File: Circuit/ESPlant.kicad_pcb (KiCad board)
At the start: 2 copper layers, 97 x 77.5 mm, 68 parts, among them P1 SOIL, P101 CONN_DIGITAL, P102 CONN_ANALOG, P103 CONN_SERIAL, P104 CONN_I2C, P105 SOLAR, P106 USB_5PIN_SHELL, P109 CONN_PWR, P110 CONN_01X05, P111 UV, P112 TEMP, P113 NEOPIXEL, P114 PIR, Q101 FDN340P, Q201 FDN340P, Q202 FDN340P, Q203 FDN340P, SW101 RESET, SW102 PRGM, SW103 RESET, U101 STM32F042F, U103 ESP-12E, U201 CN3063, U202 MCP6002, U301 BME280, U302 ADXL345

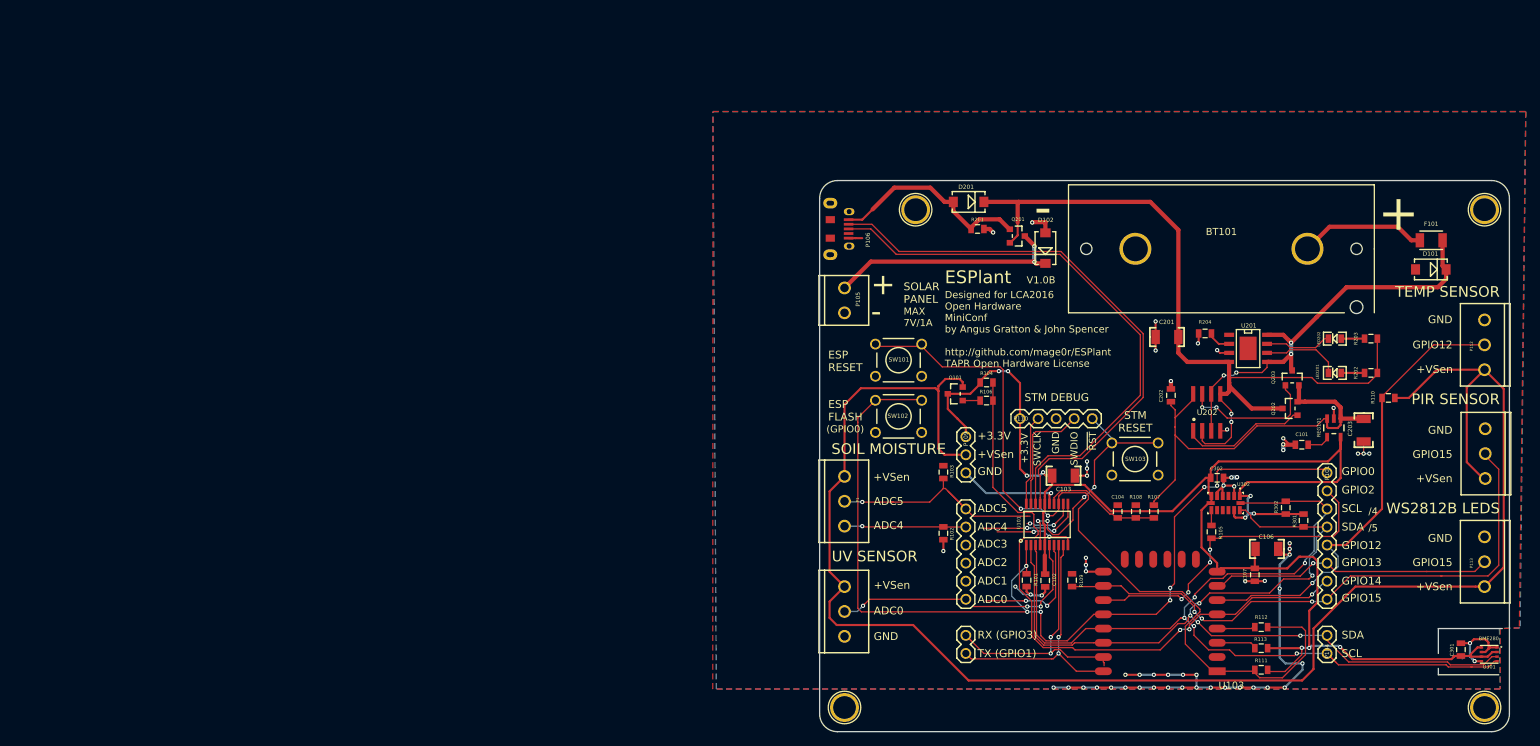
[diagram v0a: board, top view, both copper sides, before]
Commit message: Second go at a layout.
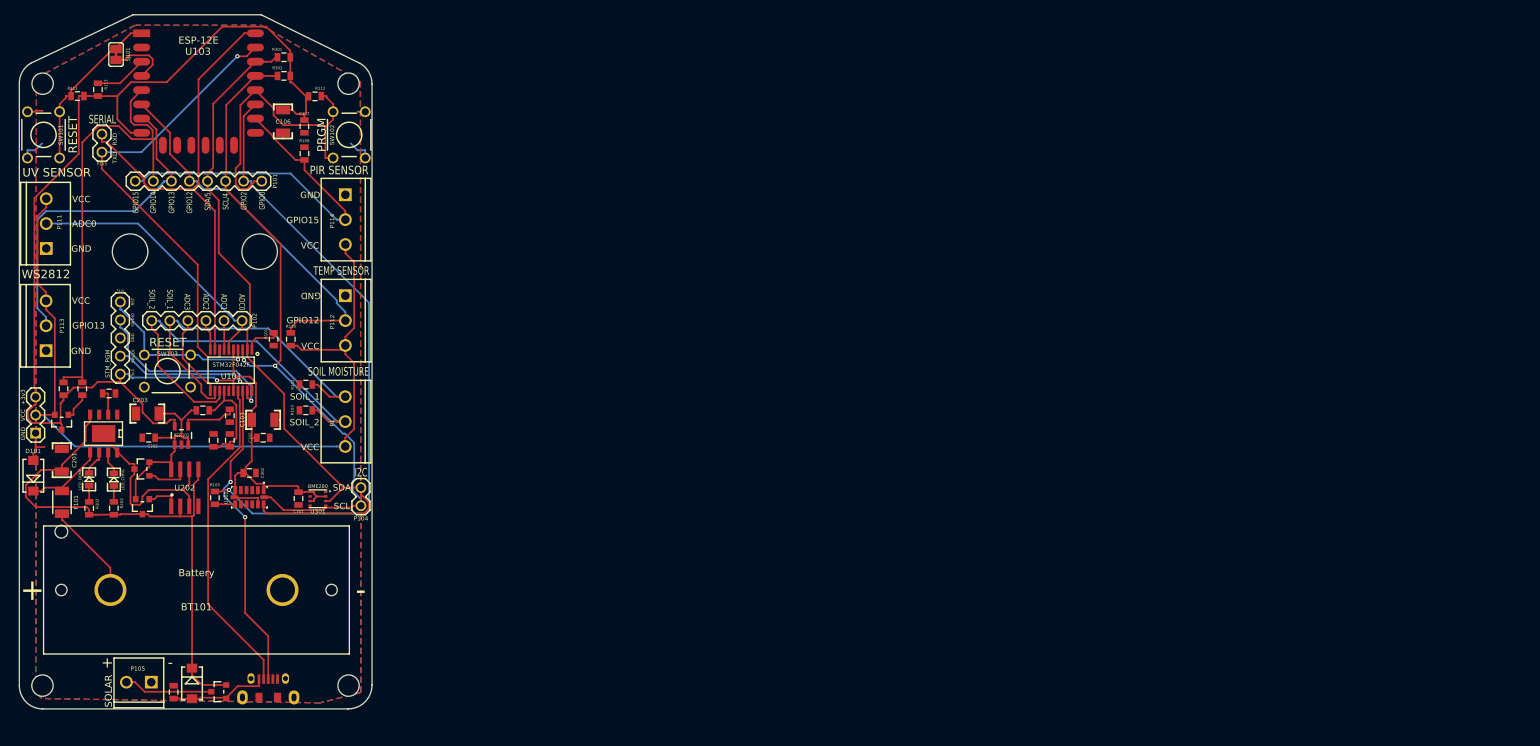
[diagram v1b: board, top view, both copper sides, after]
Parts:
- removed D102: SS14, FT:DIODE_SMA
- removed MH101, MH102, MH103, MH104: TEST_1P, Connect:1pin
- added REF01: MOUNT, Mounting_Holes:MountingHole_5mm, F.Cu at (63.3, 70.5)
- added REF03: MOUNT, Mounting_Holes:MountingHole_5mm, F.Cu at (45.0, 70.5)
- added REF05: MOUNT, Mounting_Holes:MountingHole_3mm, F.Cu at (32.7, 46.9)
- added REF06: MOUNT, Mounting_Holes:MountingHole_3mm, F.Cu at (75.8, 46.9)
- added REF07: MOUNT, Mounting_Holes:MountingHole_3mm, F.Cu at (75.8, 131.5)
- added REF08: MOUNT, Mounting_Holes:MountingHole_3mm, F.Cu at (32.7, 131.5)
- added SJ101: SJ, FT:SJ_SHORTED, F.Cu at (43.1, 42.8)
- P1: value SOIL -> SOIL MOISTURE
- P103: value CONN_SERIAL -> SERIAL
- P104: value CONN_I2C -> I2C
- P109: value CONN_PWR -> PWR
- P110: value CONN_01X05 -> STM_PGM
- P111: value UV -> UV SENSOR
- P112: value TEMP -> TEMP SENSOR
- P113: value NEOPIXEL -> WS2812
- P114: value PIR -> PIR SENSOR
- REG101: value SPX3819M5-3.3 -> SPX3819M5
- moved P113 205.0 mm to (33.2, 80.9), turned to 270 degrees
- moved D101 198.6 mm to (31.4, 102.0), turned to 270 degrees
- moved F101 196.0 mm to (35.5, 105.7), turned to 90 degrees
- moved R111 185.0 mm to (37.6, 48.6), turned to 0 degrees
- moved R113 181.5 mm to (40.5, 47.7), turned to 90 degrees
- moved R202 181.2 mm to (39.3, 106.6), turned to 90 degrees
- moved R203 178.4 mm to (42.7, 106.6), turned to 90 degrees
- moved U103 175.8 mm to (46.7, 39.8), turned to 0 degrees
- moved LED201 175.8 mm to (39.3, 102.5), turned to 90 degrees
- moved LED202 172.8 mm to (42.8, 102.6), turned to 90 degrees
- moved C203 171.1 mm to (47.5, 93.3), turned to 0 degrees
- moved U301 166.2 mm to (71.4, 105.2)
- moved C301 164.8 mm to (68.7, 105.2), turned to 270 degrees
- moved P114 163.6 mm to (75.3, 66.0)
- moved Q203 162.2 mm to (46.7, 101.1), turned to 90 degrees
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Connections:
- P102 pad 4: (no net) -> /ADC3
- P106 pad 4: (no net) -> Net-(P106-Pad4)
- R101 pad 1: /GPIO0 -> /STM_BOOT
- R111 pad 1: +3V3 -> /ESP_~RESET
- R111 pad 2: /ESP_~RESET -> +3V3
- R112 pad 1: /ESP_~RESET -> /GPIO0
- R112 pad 2: /GPIO16 -> +3V3
- U101 pad 1: /GPIO0 -> /STM_BOOT
- U101 pad 11: /SOIL_1 -> /ADC3
- U101 pad 12: /SOIL_2 -> /SOIL_1
- U101 pad 13: /ESP_~RESET -> /SOIL_2
- U103 pad 10: (no net) -> Net-(U103-Pad10)
- U103 pad 11: (no net) -> Net-(U103-Pad11)
- U103 pad 12: (no net) -> Net-(U103-Pad12)
- U103 pad 13: (no net) -> Net-(U103-Pad13)
- U103 pad 14: (no net) -> Net-(U103-Pad14)
- U103 pad 2: (no net) -> Net-(U103-Pad2)
- U103 pad 9: (no net) -> Net-(U103-Pad9)
- U302 pad 10: (no net) -> Net-(U302-Pad10)
- U302 pad 11: (no net) -> Net-(U302-Pad11)
- U302 pad 3: (no net) -> Net-(U302-Pad3)
- U302 pad 9: (no net) -> Net-(U302-Pad9)
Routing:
- net GND: track 154.1 -> 15.6 mm, vias 62 -> 0
- net /VCC_SENS: track 234.0 -> 118.3 mm
- net /GPIO0: track 136.4 -> 42.8 mm, vias 7 -> 0
- net /ESP_~RESET: track 114.6 -> 24.4 mm, vias 2 -> 0
- net /GPIO2: track 46.9 -> 88.9 mm, vias 4 -> 1
- net /Power/VIN: track 116.6 -> 78.4 mm, vias 2 -> 0
- net /USB_D+: track 79.7 -> 44.2 mm, vias 0 -> 2
- net /USB_D-: track 80.6 -> 45.7 mm
- net /Power/VOUT: track 62.4 -> 28.1 mm
- net /I2C Sensors/I2C_SCL: track 128.5 -> 95.3 mm, vias 5 -> 2
- net /STM_RXD: track 36.5 -> 67.3 mm, vias 2 -> 0
- net /GPIO15: track 82.1 -> 53.0 mm, vias 3 -> 0
- net /I2C Sensors/I2C_SDA: track 125.8 -> 99.6 mm, vias 5 -> 0
- net /STM_TXD: track 39.3 -> 65.4 mm, vias 2 -> 1
- net +3V3: track 225.6 -> 201.3 mm, vias 10 -> 1
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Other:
- board size 97 x 77.5 mm -> 49.6 x 97.6 mm
- net class Default: clearance 0.15 -> 0.2; trace_width 0.15 -> 0.25; via_drill 0.3 -> 0.4
- net class Power removed
- net class USB removed
- rule trace_clearance: 0.15 -> 0.2
- rule trace_min: 0.15 -> 0.2
- board text added: "+3v3"
- board text added: "ESPlant - Version 1.0 https://github.com/mage0r/ESPlant Designed by: John Spencer and Angus Gratton Open Hardware MiniConf, LinuxConf, Geelong, 2016 Made at hackmelbourne.org"
- board text added: "I2C"
- board text added: "PWR"
- board text added: "RST"
- board text added: "RXD"
- board text added: "SCL/4"
- board text added: "SDA/5"
- board text added: "SERIAL"
- board text added: "SOIL_1"
- board text added: "SOIL_2"
- board text added: "SOLAR"
- board text added: "STM_PGM"
- board text added: "TXD"
- board text added: "VCC"
- board text added: "WS2812"
- board text removed: "(GPIO0)"
- board text removed: "+3.3V"
- board text removed: "+VSen"
- board text removed: "/4"
- board text removed: "/5"
- board text removed: "ADC4"
- board text removed: "ADC5"
- board text removed: "Designed for LCA2016 Open Hardware MiniConf by Angus Gratton & John Spencer http://github.com/mage0r/ESPlant TAPR Open Hardware License"
- board text removed: "ESP FLASH"
- board text removed: "ESP RESET"
- board text removed: "ESPlant"
- board text removed: "MAX 7V/1A"
- board text removed: "RX (GPIO3)"
- board text removed: "SOLAR PANEL"
- board text removed: "STM DEBUG"
- board text removed: "STM RESET"
- board text removed: "TX (GPIO1)"
- board text removed: "V1.0B"
- board text removed: "WS2812B LEDS"
- board text removed: "~RST"
